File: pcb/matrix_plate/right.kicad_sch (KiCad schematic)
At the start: 23 parts

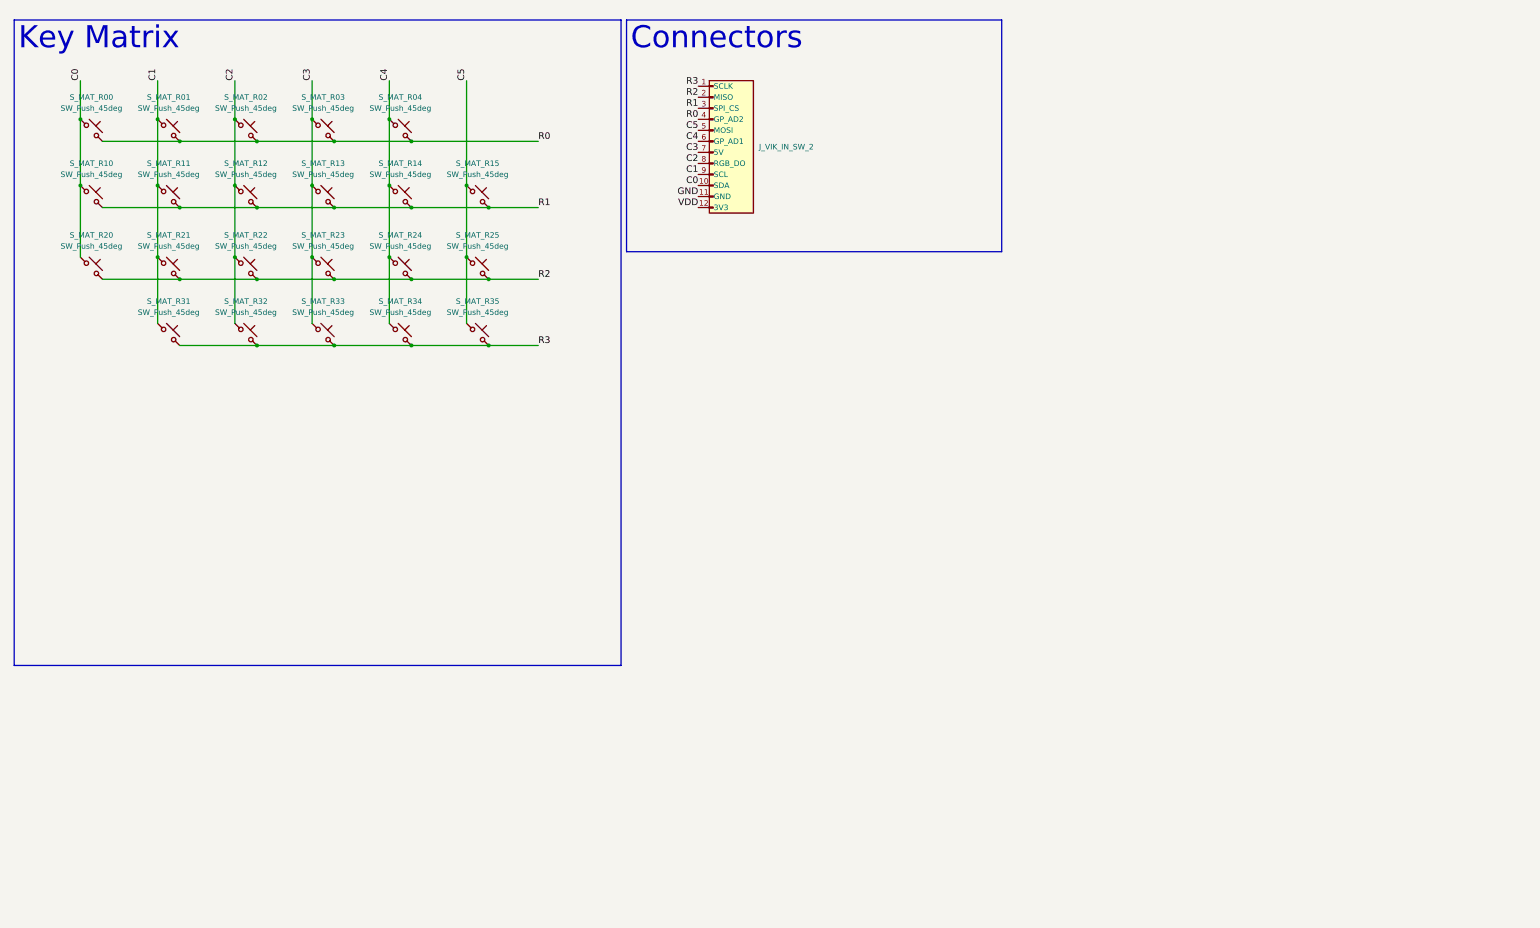
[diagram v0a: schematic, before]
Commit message: Work on PCBs.
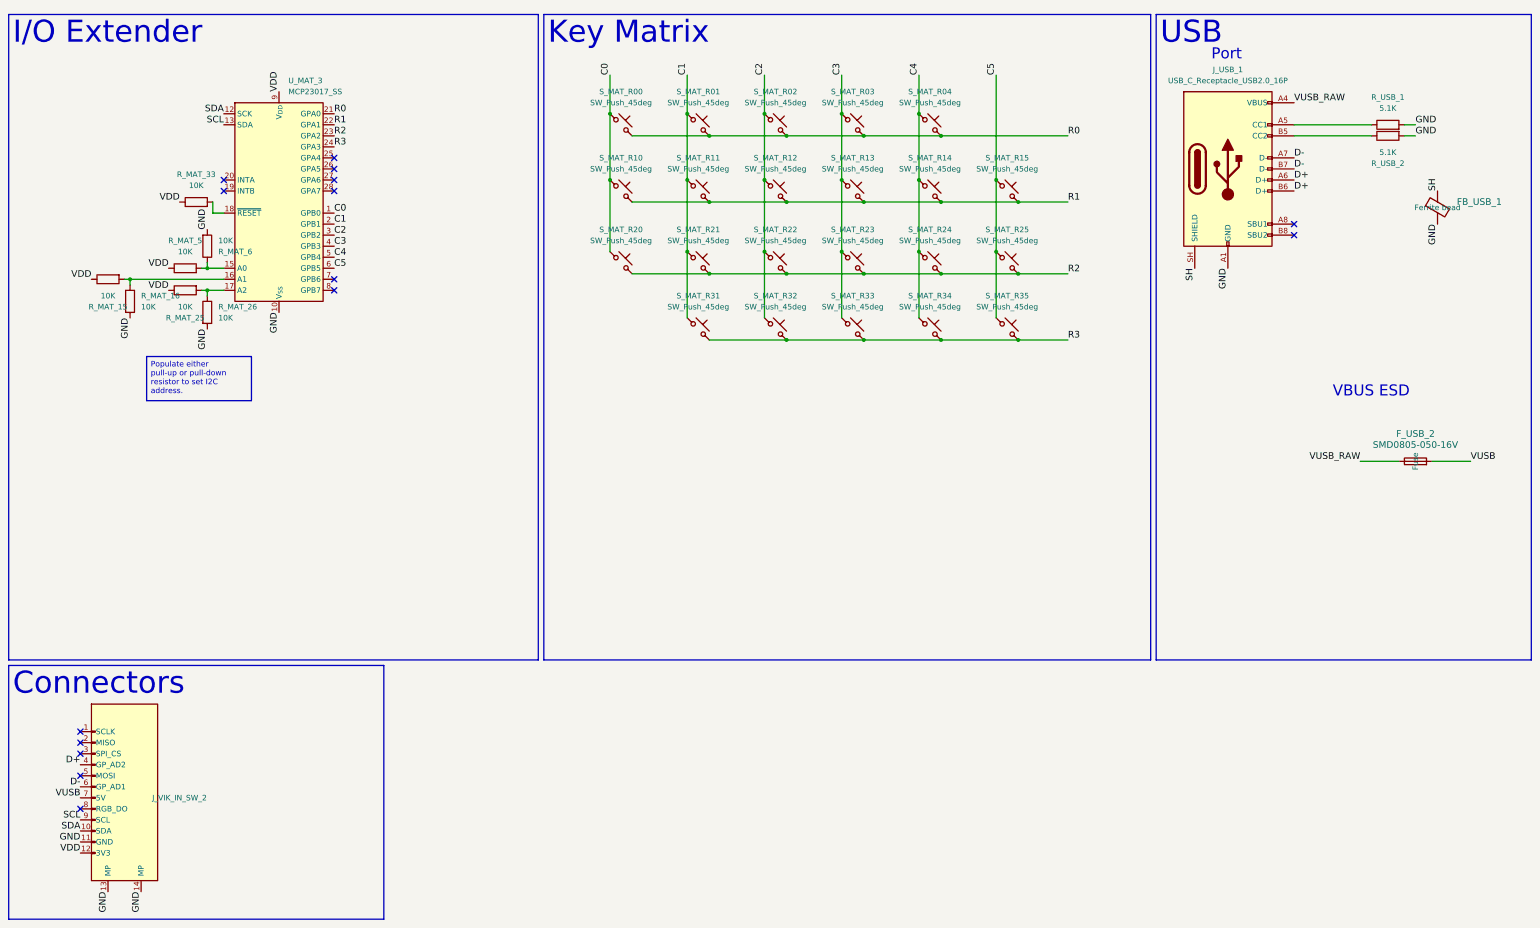
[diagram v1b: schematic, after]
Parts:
- added FB_USB_1: (no value), Inductor_SMD:L_0805_2012Metric, symbol Device:FerriteBead
- added F_USB_2: SMD0805-050-16V, Fuse:Fuse_0805_2012Metric, symbol Device:Fuse
- added J_USB_1: USB_C_Receptacle_USB2.0_16P, Connector_USB:USB_C_Receptacle_HRO_TYPE-C-31-M-12, symbol Connector:USB_C_Receptacle_USB2.0_16P
- added R_MAT_15, R_MAT_16, R_MAT_25, R_MAT_26, R_MAT_33, R_MAT_5, R_MAT_6: 10K, Resistor_SMD:R_0201_0603Metric_Pad0.64x0.40mm_HandSolder, symbol Device:R
- added R_USB_1, R_USB_2: 5.1K, Resistor_SMD:R_0201_0603Metric_Pad0.64x0.40mm_HandSolder, symbol Device:R
- added U_MAT_3: MCP23017_SS, Package_SO:SSOP-28_5.3x10.2mm_P0.65mm, symbol Interface_Expansion:MCP23017x-x-SS
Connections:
- net C0: now also U_MAT_3.1 (GPB0); no longer J_VIK_IN_SW_2.10 (SDA)
- net C1: now also U_MAT_3.2 (GPB1); no longer J_VIK_IN_SW_2.9 (SCL)
- net C2: now also U_MAT_3.3 (GPB2); no longer J_VIK_IN_SW_2.8 (RGB_DO)
- net C3: now also U_MAT_3.4 (GPB3); no longer J_VIK_IN_SW_2.7 (5V)
- net C4: now also U_MAT_3.5 (GPB4); no longer J_VIK_IN_SW_2.6 (GP_AD1)
- net C5: now also U_MAT_3.6 (GPB5); no longer J_VIK_IN_SW_2.5 (MOSI)
- net GND: now also J_VIK_IN_SW_2.13 (MP), J_VIK_IN_SW_2.14 (MP), FB_USB_1.2, J_USB_1.A1 (GND), J_USB_1.A12 (GND), J_USB_1.B1 (GND), J_USB_1.B12 (GND), R_MAT_16.2, R_MAT_26.2, R_MAT_6.2, R_USB_1.2, R_USB_2.2, U_MAT_3.10 (V_{SS})
- net R0: now also U_MAT_3.21 (GPA0); no longer J_VIK_IN_SW_2.4 (GP_AD2)
- net R1: now also U_MAT_3.22 (GPA1); no longer J_VIK_IN_SW_2.3 (SPI_CS)
- net R2: now also U_MAT_3.23 (GPA2); no longer J_VIK_IN_SW_2.2 (MISO)
- net R3: now also U_MAT_3.24 (GPA3); no longer J_VIK_IN_SW_2.1 (SCLK)
- net VDD: now also R_MAT_15.1, R_MAT_25.1, R_MAT_33.1, R_MAT_5.1, U_MAT_3.9 (V_{DD})
- new net: J_USB_1.A5 (CC1), R_USB_1.1
- new net: J_USB_1.B5 (CC2), R_USB_2.1
- new net: R_MAT_15.2, R_MAT_16.1, U_MAT_3.16 (A1)
- new net: R_MAT_25.2, R_MAT_26.1, U_MAT_3.17 (A2)
- new net: R_MAT_5.2, R_MAT_6.1, U_MAT_3.15 (A0)
- new net: R_MAT_33.2, U_MAT_3.18 (~{RESET})
- new net D+: J_USB_1.A6 (D+), J_USB_1.B6 (D+), J_VIK_IN_SW_2.4 (GP_AD2)
- new net D-: J_USB_1.A7 (D-), J_USB_1.B7 (D-), J_VIK_IN_SW_2.6 (GP_AD1)
- new net SCL: J_VIK_IN_SW_2.9 (SCL), U_MAT_3.13 (SDA)
- new net SDA: J_VIK_IN_SW_2.10 (SDA), U_MAT_3.12 (SCK)
- new net SH: FB_USB_1.1, J_USB_1.SH (SHIELD)
- new net VUSB: F_USB_2.2, J_VIK_IN_SW_2.7 (5V)
- new net VUSB_RAW: F_USB_2.1, J_USB_1.A4 (VBUS), J_USB_1.A9 (VBUS), J_USB_1.B4 (VBUS), J_USB_1.B9 (VBUS)
- no-connect marks 0 -> 15
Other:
- note added: "Port"
- note added: "VBUS ESD"
- moved on the sheet: S_MAT_R00, S_MAT_R01, S_MAT_R02, S_MAT_R03, S_MAT_R04, S_MAT_R10, S_MAT_R11, S_MAT_R12, S_MAT_R13, S_MAT_R14, S_MAT_R15, S_MAT_R20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
